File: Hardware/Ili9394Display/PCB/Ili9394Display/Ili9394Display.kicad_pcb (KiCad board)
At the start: 2 copper layers, 27.9 x 27.9 mm, 2 parts, among them J1 Conn_01x08_Male, J2 Conn_01x08_Female

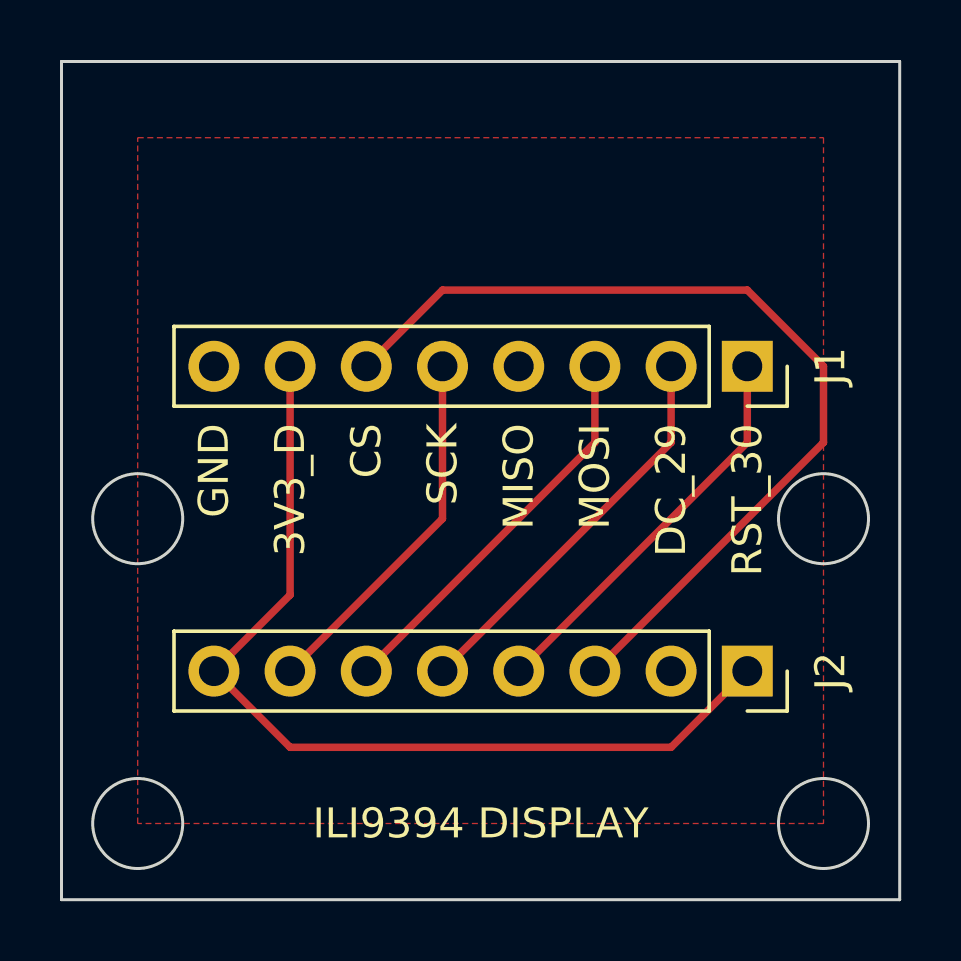
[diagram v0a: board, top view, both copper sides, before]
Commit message: Finalised PCBs
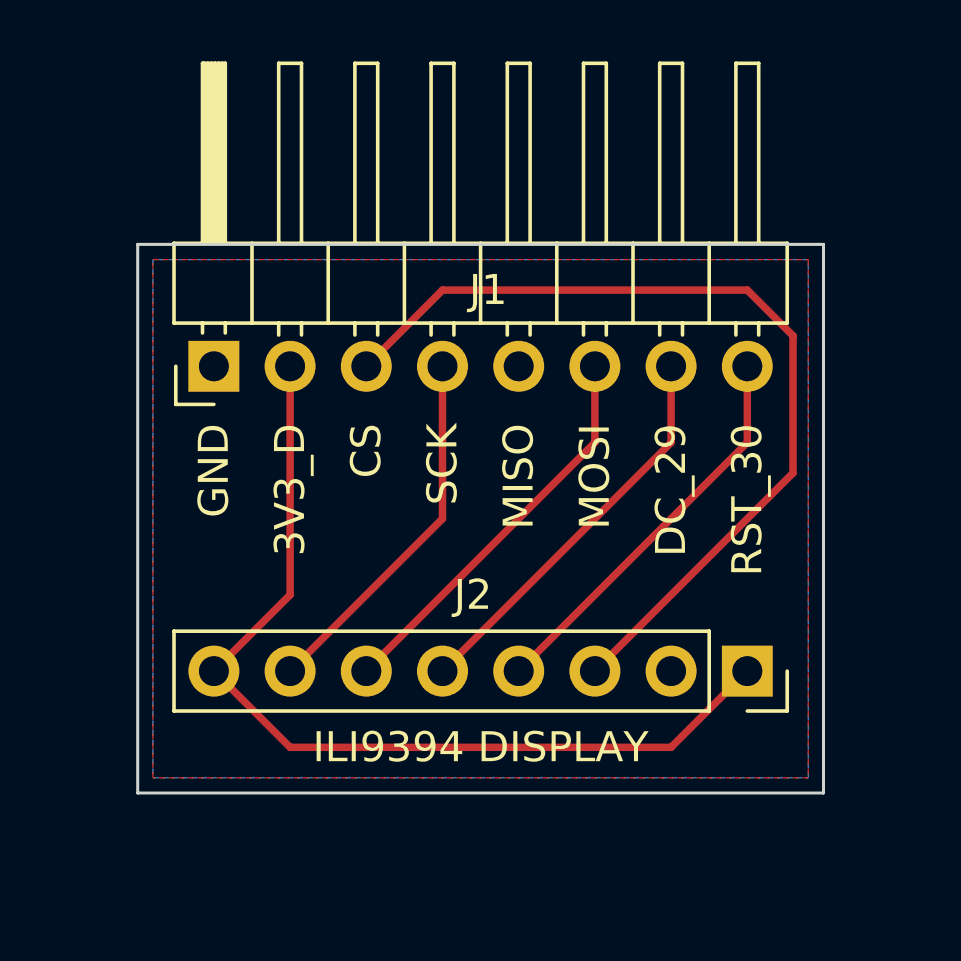
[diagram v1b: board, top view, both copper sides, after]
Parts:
- J1: footprint Connector_PinSocket_2.54mm:PinSocket_1x08_P2.54mm_Vertical -> Connector_PinHeader_2.54mm:PinHeader_1x08_P2.54mm_Horizontal
- moved J1 17.8 mm to (71.1, 53.3), turned to 90 degrees
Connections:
- J1 pad 1: RST -> GND
- J1 pad 2: DC -> 3V3_D
- J1 pad 3: MOSI -> CS
- J1 pad 4: MISO -> SCK
- J1 pad 5: SCK -> MISO
- J1 pad 6: CS -> MOSI
- J1 pad 7: 3V3_D -> DC
- J1 pad 8: GND -> RST
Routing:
- net CS: track 30.7 -> 29.8 mm
- added copper zone on B.Cu, net GND
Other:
- board size 27.9 x 27.9 mm -> 22.9 x 18.3 mm
